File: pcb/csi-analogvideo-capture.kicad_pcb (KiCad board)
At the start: 2 copper layers, 55 x 50 mm, 69 parts, among them CN1 rpi_camera_conn_top, J1 ANALOG_IN, U1 BD18KA5FP-E2, U2 ADV7280A-M, Y1 ABM8G-28.63636MHZ

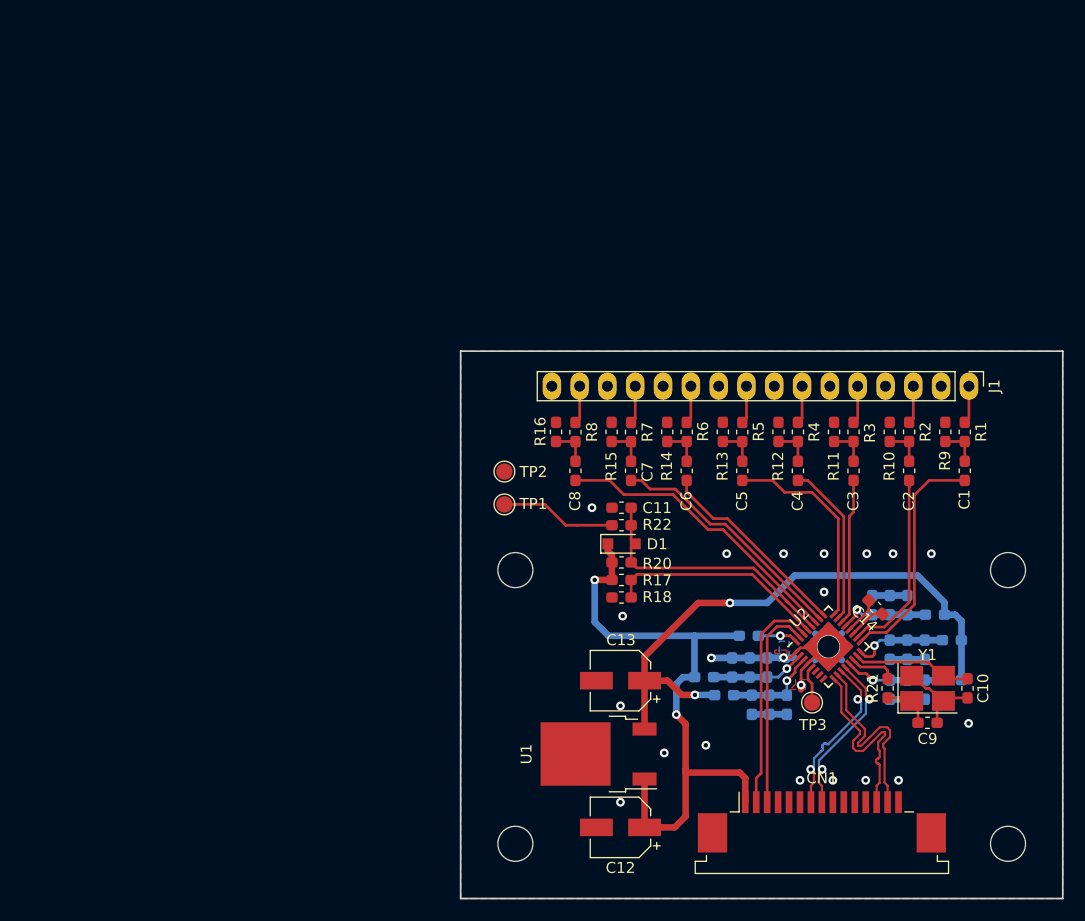
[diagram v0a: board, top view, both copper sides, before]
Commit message: update schematicand pcb, DRC passed
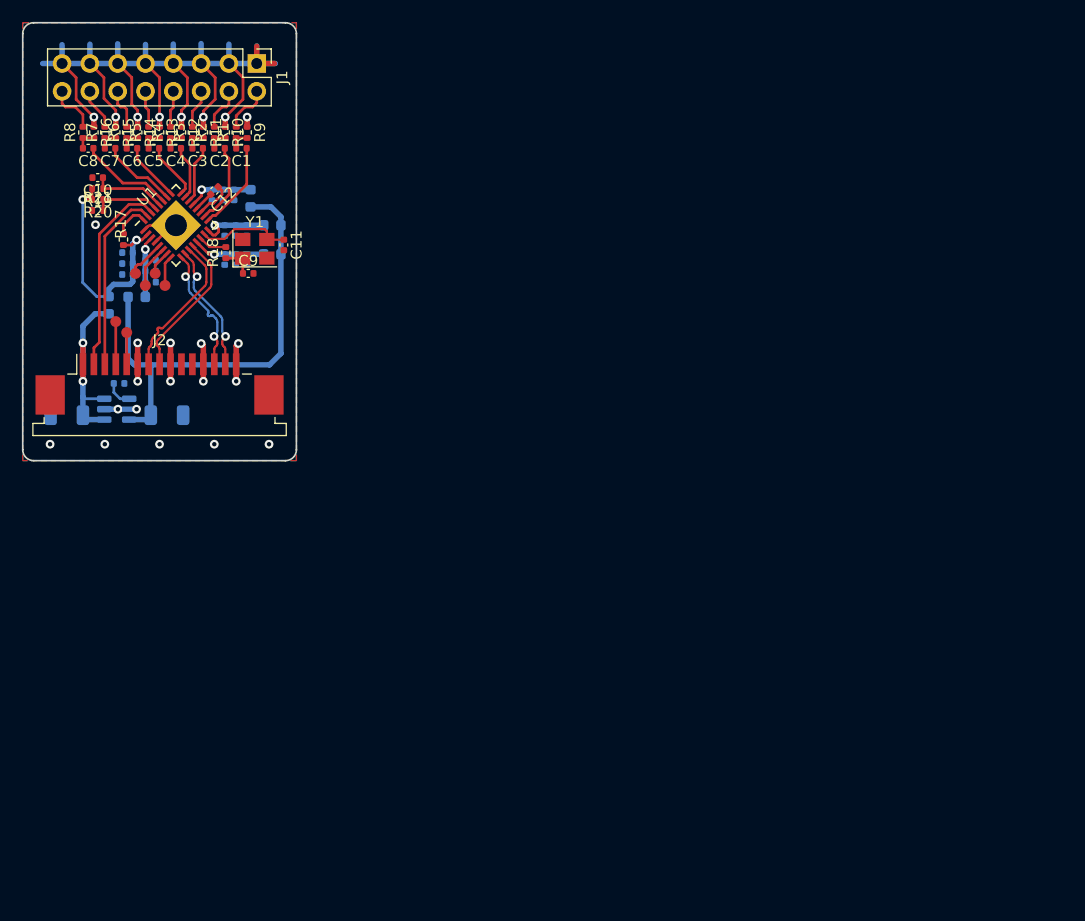
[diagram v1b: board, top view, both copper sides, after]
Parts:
- removed CN1: rpi_camera_conn_top, Connector_FFC-FPC:TE_1-84953-5_1x15-1MP_P1.0mm_Horizontal
- removed D1: D, Diode_SMD:D_SOD-323_HandSoldering
- removed H1, H2, H3, H4: MountingHole, MountingHole:MountingHole_3.2mm_M3_ISO14580
- removed L1, L2, L3, L4, L5: FB, Inductor_SMD:L_0603_1608Metric_Pad1.05x0.95mm_HandSolder
- removed R22: 47Ω, Resistor_SMD:R_0603_1608Metric_Pad1.05x0.95mm_HandSolder
- added C30: 10nF, Capacitor_SMD:C_0402_1005Metric, B.Cu at (68.5, 59.0)
- added FB1: 600Ω, Inductor_SMD:L_0603_1608Metric, B.Cu at (57.9, 65.8)
- added FB2: 600Ω, Inductor_SMD:L_0603_1608Metric, B.Cu at (60.4, 65.0)
- added FB3: 600Ω, Inductor_SMD:L_0603_1608Metric, B.Cu at (70.8, 56.0)
- added FB4: 600Ω, Inductor_SMD:L_0603_1608Metric, B.Cu at (72.8, 61.1)
- added FB5: 600Ω, Inductor_SMD:L_0603_1608Metric, B.Cu at (72.8, 58.5)
- added J2: rpi_camera_conn_top, Connector_FFC-FPC:TE_1-84953-5_1x15-1MP_P1.0mm_Horizontal, F.Cu at (62.5, 73.0)
- added TP4: TestPoint, TestPoint:TestPoint_Pad_D1.0mm, F.Cu at (63.0, 64.0)
- added TP5: TestPoint, TestPoint:TestPoint_Pad_D1.0mm, F.Cu at (59.5, 68.3)
- added TP6: TestPoint, TestPoint:TestPoint_Pad_D1.0mm, F.Cu at (58.5, 67.3)
- C1, C16, C17, C18, C19, C2, C21, C22, C23, C24, C26, C27, C28, C29, C3, C4, C5, C6, C7, C8, C9: footprint Capacitor_SMD:C_0603_1608Metric_Pad1.05x0.95mm_HandSolder -> Capacitor_SMD:C_0402_1005Metric
- C10: value 20pF -> 4.7μF; footprint Capacitor_SMD:C_0603_1608Metric_Pad1.05x0.95mm_HandSolder -> Capacitor_SMD:C_0402_1005Metric
- C11: value 2.2μF -> 20pF; footprint Capacitor_SMD:C_0603_1608Metric_Pad1.05x0.95mm_HandSolder -> Capacitor_SMD:C_0402_1005Metric
- C12: value 47μF -> 0.1μF; footprint Capacitor_SMD:CP_Elec_5x5.3 -> Capacitor_SMD:C_0402_1005Metric
- C13: value 47μF -> 100μF; footprint Capacitor_SMD:CP_Elec_5x5.3 -> Capacitor_SMD:C_1206_3216Metric; moved to B.Cu
- C14: value 0.1μF -> 10nF; footprint Capacitor_SMD:C_0603_1608Metric_Pad1.05x0.95mm_HandSolder -> Capacitor_SMD:C_0402_1005Metric; moved to B.Cu
- C15: value 10μF -> 47μF; footprint Capacitor_SMD:C_0603_1608Metric_Pad1.05x0.95mm_HandSolder -> Capacitor_SMD:C_1206_3216Metric
- C20: value 0.1μF -> 10μF; footprint Capacitor_SMD:C_0603_1608Metric_Pad1.05x0.95mm_HandSolder -> Capacitor_SMD:C_0402_1005Metric
- C25: value 10nF -> 0.1μF; footprint Capacitor_SMD:C_0603_1608Metric_Pad1.05x0.95mm_HandSolder -> Capacitor_SMD:C_0402_1005Metric
- J1: value ANALOG_IN -> VIDEO_IN; footprint Connector_PinHeader_2.54mm:PinHeader_1x16_P2.54mm_Vertical -> Connector_PinHeader_2.54mm:PinHeader_2x08_P2.54mm_Vertical
- R1, R10, R11, R12, R13, R14, R15, R16, R17, R2, R20, R3, R4, R5, R6, R7, R8, R9: footprint Resistor_SMD:R_0603_1608Metric_Pad1.05x0.95mm_HandSolder -> Resistor_SMD:R_0402_1005Metric
- R18: value NI -> 560Ω; footprint Resistor_SMD:R_0603_1608Metric_Pad1.05x0.95mm_HandSolder -> Resistor_SMD:R_0402_1005Metric
- R19: footprint Resistor_SMD:R_0603_1608Metric_Pad1.05x0.95mm_HandSolder -> Resistor_SMD:R_0402_1005Metric; moved to F.Cu
- R21: value 560Ω -> DNP; footprint Resistor_SMD:R_0603_1608Metric_Pad1.05x0.95mm_HandSolder -> Resistor_SMD:R_0402_1005Metric
- TP1: value ~{RESET} -> TestPoint; footprint TestPoint:TestPoint_Pad_D1.5mm -> TestPoint:TestPoint_Pad_D1.0mm
- TP2: value GND -> TestPoint; footprint TestPoint:TestPoint_Pad_D1.5mm -> TestPoint:TestPoint_Pad_D1.0mm
- TP3: value ~{INTRQ} -> TestPoint; footprint TestPoint:TestPoint_Pad_D1.5mm -> TestPoint:TestPoint_Pad_D1.0mm
- U1: value BD18KA5FP-E2 -> ADV7280A-M; footprint Package_TO_SOT_SMD:TO-252-2 -> Package_CSP:LFCSP-32-1EP_5x5mm_P0.5mm_EP3.25x3.25mm
- U2: value ADV7280A-M -> NJM12888F18; footprint Package_CSP:LFCSP-32-1EP_5x5mm_P0.5mm_EP3.25x3.25mm -> Package_TO_SOT_SMD:SOT-23-5; moved to B.Cu
- Y1: footprint Crystal:Crystal_SMD_3225-4Pin_3.2x2.5mm_HandSoldering -> Crystal:Crystal_SMD_3225-4Pin_3.2x2.5mm
- moved C10 92.1 mm to (56.9, 54.1), turned to 180 degrees
- moved R21 84.3 mm to (56.9, 57.1), turned to 0 degrees
- moved C18 77.6 mm to (69.3, 55.7)
- moved C23 77.1 mm to (68.3, 55.7)
- moved C28 76.6 mm to (67.3, 55.7)
- moved C17 75.2 mm to (61.7, 63.7), turned to 0 degrees
- moved C9 74.4 mm to (70.6, 62.9)
- moved C22 74.1 mm to (61.7, 62.7), turned to 0 degrees
- moved Y1 73.4 mm to (71.2, 60.6)
- moved C27 73.1 mm to (61.7, 61.7), turned to 0 degrees
- moved C26 73.0 mm to (59.6, 61.0), turned to 180 degrees
- moved C1 72.3 mm to (70.0, 51.5), turned to 180 degrees
- moved R19 72.2 mm to (56.9, 55.1)
- moved C14 72.1 mm to (58.8, 73.0), turned to 0 degrees
- moved R1 72.0 mm to (69.5, 50.0)
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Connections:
- C10 pad 1: Net-(C10-Pad1) -> /~{RESET}
- C11 pad 1: Net-(C11-Pad1) -> /XTALN
- C12 pad 1: +3V3 -> Net-(C12-Pad1)
- C12 pad 2: GND -> Net-(C12-Pad2)
- C13 pad 1: +1V8 -> +3V3
- C14 pad 2: Net-(C14-Pad2) -> GND
- C15 pad 1: /DVDDIO_3V3 -> +1V8
- C16 pad 1: /DVDD_1V8 -> /DVDDIO_3V3
- C17 pad 1: /AVDD_1V8 -> /DVDD_1V8
- C18 pad 1: /MVDD_1V8 -> /AVDD_1V8
- C19 pad 1: /PVDD_1V8 -> /MVDD_1V8
- C20 pad 1: /DVDDIO_3V3 -> /PVDD_1V8
- C21 pad 1: /DVDD_1V8 -> /DVDDIO_3V3
- C22 pad 1: /AVDD_1V8 -> /DVDD_1V8
- C23 pad 1: /MVDD_1V8 -> /AVDD_1V8
- C24 pad 1: /PVDD_1V8 -> /MVDD_1V8
- C25 pad 1: /DVDDIO_3V3 -> /PVDD_1V8
- C26 pad 1: /DVDD_1V8 -> /DVDDIO_3V3
- C27 pad 1: /AVDD_1V8 -> /DVDD_1V8
- C28 pad 1: /MVDD_1V8 -> /AVDD_1V8
- C29 pad 1: /PVDD_1V8 -> /MVDD_1V8
- J1 pad 1: /P_AIN1 -> GND
- J1 pad 10: GND -> /VIN5
- J1 pad 11: /P_AIN6 -> GND
- J1 pad 12: GND -> /VIN6
- J1 pad 13: /P_AIN7 -> GND
- J1 pad 14: GND -> /VIN7
- J1 pad 15: /P_AIN8 -> GND
- J1 pad 16: GND -> /VIN8
- J1 pad 2: GND -> /VIN1
- J1 pad 3: /P_AIN2 -> GND
- J1 pad 4: GND -> /VIN2
- J1 pad 5: /P_AIN3 -> GND
- J1 pad 6: GND -> /VIN3
- J1 pad 7: /P_AIN4 -> GND
- J1 pad 8: GND -> /VIN4
- J1 pad 9: /P_AIN5 -> GND
- R1 pad 2: /P_AIN1 -> /VIN1
- R10 pad 1: Net-(C2-Pad2) -> GND
- R10 pad 2: GND -> Net-(C2-Pad2)
- R12 pad 1: Net-(C4-Pad2) -> GND
- R12 pad 2: GND -> Net-(C4-Pad2)
- R14 pad 1: Net-(C6-Pad2) -> GND
- R14 pad 2: GND -> Net-(C6-Pad2)
- R16 pad 1: Net-(C8-Pad2) -> GND
- R16 pad 2: GND -> Net-(C8-Pad2)
- R17 pad 1: Net-(R17-Pad1) -> /~{PWRDWN}
- R17 pad 2: +3V3 -> /DVDDIO_3V3
- R18 pad 1: GND -> Net-(C9-Pad1)
- R18 pad 2: Net-(R17-Pad1) -> /XTALP
- R19 pad 1: Net-(R19-Pad1) -> /~{RESET}
- R19 pad 2: +3V3 -> /DVDDIO_3V3
- R2 pad 2: /P_AIN2 -> /VIN2
- R20 pad 1: Net-(C11-Pad1) -> /ALSB
- R20 pad 2: +3V3 -> /DVDDIO_3V3
- R21 pad 1: Net-(R21-Pad1) -> GND
- R21 pad 2: Net-(C9-Pad1) -> /ALSB
- R3 pad 2: /P_AIN3 -> /VIN3
- R4 pad 2: /P_AIN4 -> /VIN4
- R5 pad 2: /P_AIN5 -> /VIN5
- R6 pad 2: /P_AIN6 -> /VIN6
- R7 pad 2: /P_AIN7 -> /VIN7
- R8 pad 2: /P_AIN8 -> /VIN8
- TP1 pad 1: Net-(R22-Pad2) -> /~{INTRQ}
- TP2 pad 1: GND -> /GPO2
- TP3 pad 1: Net-(TP3-Pad1) -> /GPO1
- U1 pad 1: +3V3 -> GND
- U1 pad 2: GND -> /DVDDIO_3V3
- U1 pad 3: +1V8 -> /DVDD_1V8
- U2 pad 1: GND -> +3V3
- U2 pad 2: /DVDDIO_3V3 -> GND
- U2 pad 3: /DVDD_1V8 -> +3V3
- U2 pad 4: GND -> Net-(C14-Pad1)
- U2 pad 5: Net-(TP3-Pad1) -> +1V8
- Y1 pad 3: Net-(C10-Pad1) -> /XTALN
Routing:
- net GND: track 45.3 -> 108.8 mm, vias 22 -> 24
- net +3V3: track 57.2 -> 18.6 mm
- net Net-(C11-Pad1): track 24.4 -> 0.00 mm
- net Net-(R17-Pad1): track 20.1 -> 0.00 mm
- net /AIN8: track 27.3 -> 8.65 mm
- net /AIN7: track 22.4 -> 6.97 mm
- net /AIN5: track 19.2 -> 5.25 mm
- net /DVDDIO_3V3: track 8.71 -> 22.1 mm, vias 1 -> 2
- net /AIN1: track 21.5 -> 8.18 mm
- net /AIN6: track 18.2 -> 5.37 mm
- net Net-(C10-Pad1): track 11.0 -> 0.00 mm
- net +1V8: track 53.4 -> 42.6 mm, vias 2 -> 0
- net Net-(R22-Pad2): track 10.6 -> 0.00 mm
- net /AIN4: track 15.1 -> 4.98 mm
- net /AIN2: track 17.3 -> 7.48 mm
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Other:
- board size 55 x 50 mm -> 25 x 40 mm
- rule pad_to_mask_clearance: 0.2 -> 0
